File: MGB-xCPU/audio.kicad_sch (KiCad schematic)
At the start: 39 parts, among them P5 Headphones, U3 IR3R53N

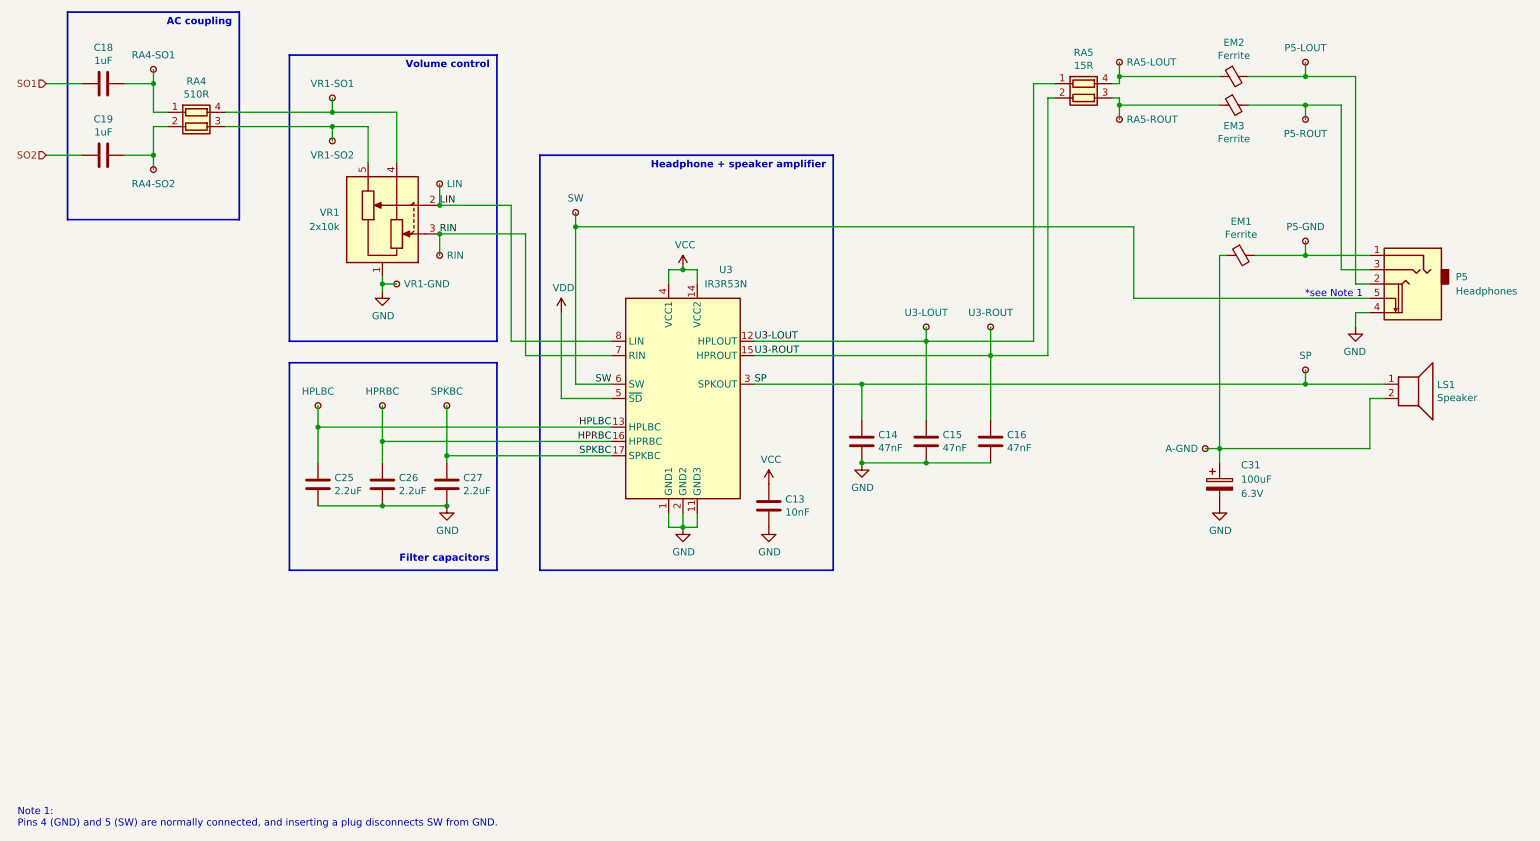
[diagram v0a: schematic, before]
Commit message: Update to latest KiCad
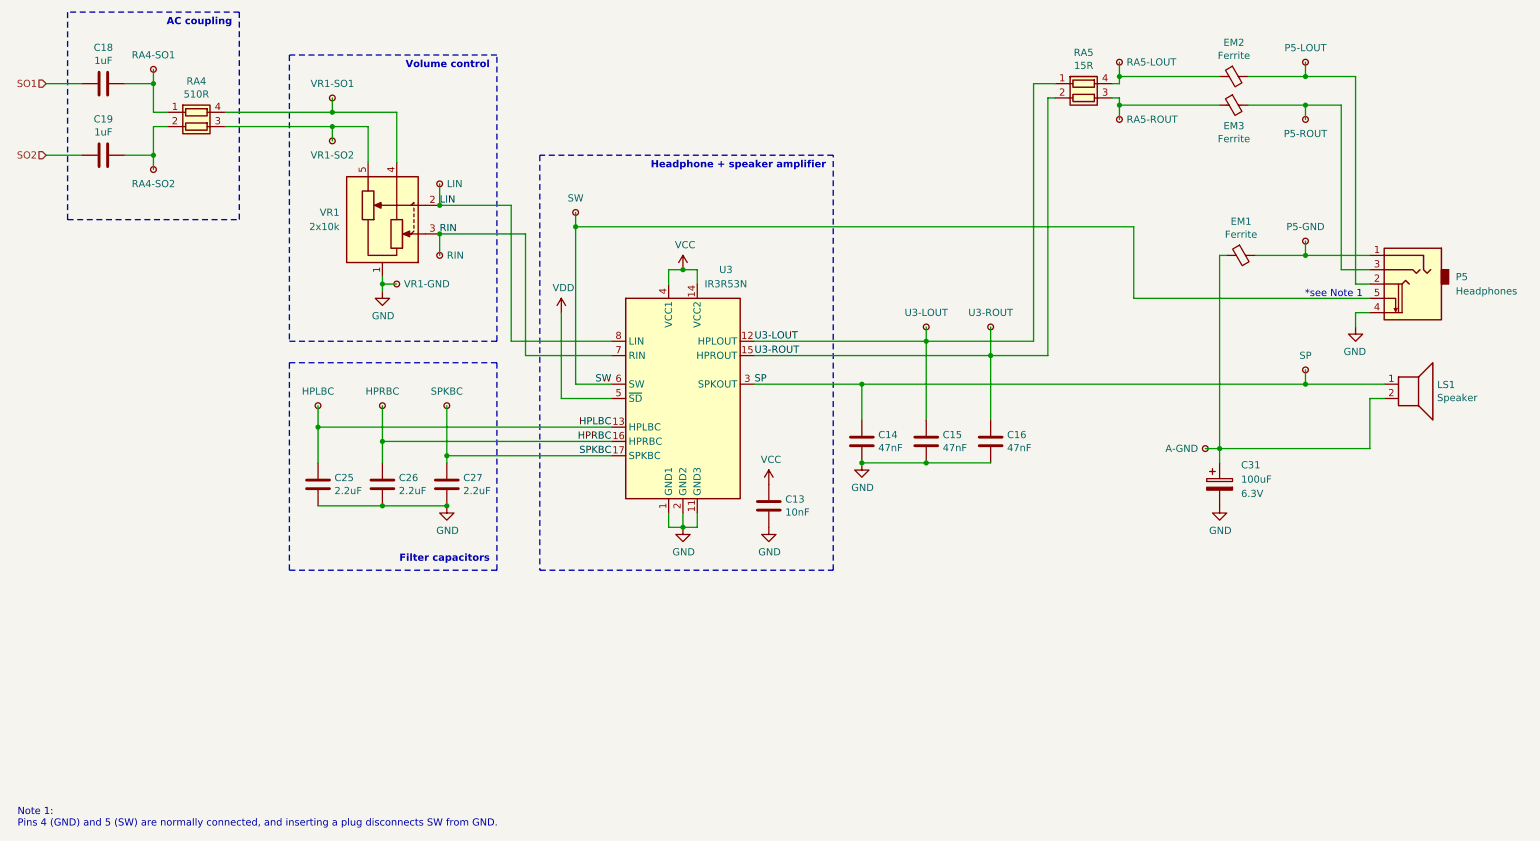
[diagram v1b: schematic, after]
